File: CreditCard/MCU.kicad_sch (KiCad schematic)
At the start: 20 parts, among them J2 MEM2052-00-195-00-A_REVA, U3 PTS645SK43SMTR92LFS, U4 PTS645SK43SMTR92LFS, U8 ESP32-C6-WROOM-1U-N4, Y1 MS1V-T1K-32.768KHZ-12.5PF-20P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

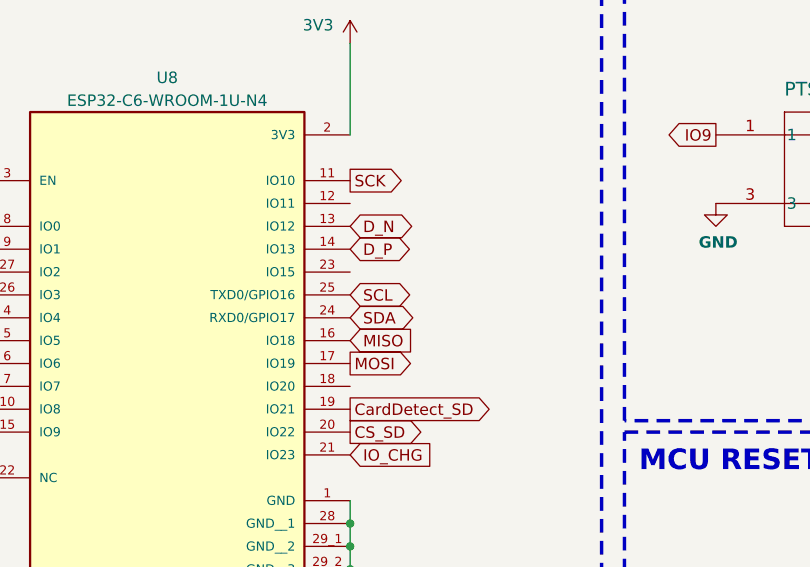
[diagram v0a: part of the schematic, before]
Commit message: connection du audio amp
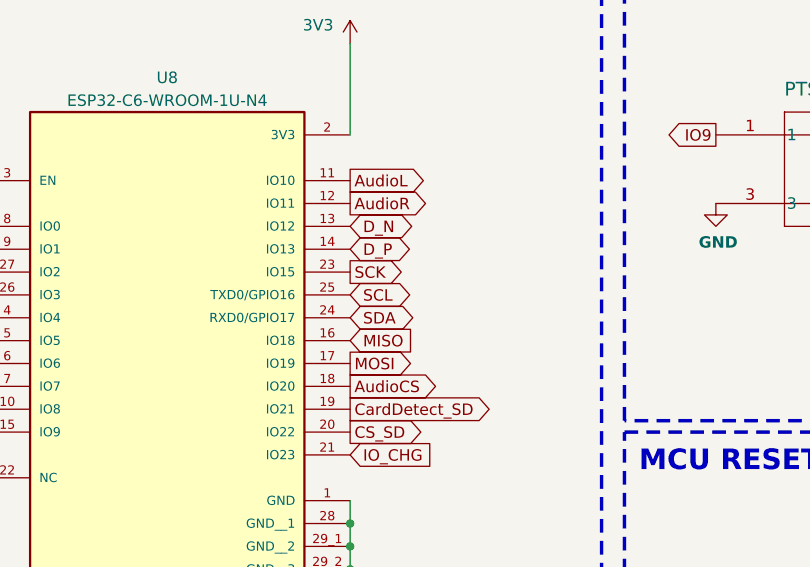
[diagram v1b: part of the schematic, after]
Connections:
- net SCK: now also U8.23 (IO15); no longer U8.11 (IO10)
- net AudioR: now reaches U8.12 (IO11)
- net AudioCS: now reaches U8.18 (IO20)
- new net AudioL: U8.11 (IO10)
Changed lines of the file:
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@@
+		)
+	)
+	(global_label "AudioL"
+		(shape output)
+		(at 185.42 48.26 0)
+		(fields_autoplaced yes)
+		(effects
+			(font
+				(size 1.27 1.27)
+			)
+			(justify left)
+		)
+		(property "Intersheetrefs" "${INTERSHEET_REFS}"
+			(at 194.5737 48.26 0)
+			(effects
+				(font
+					(size 1.27 1.27)
+				)
+				(justify left)
+				(hide yes)
+			)
 		)
 	)
@@
 		)
 	)
+	(global_label "SCK"
+		(shape output)
+		(at 185.42 58.42 0)
+		(fields_autoplaced yes)
+		(effects
+			(font
+				(size 1.27 1.27)
+			)
+			(justify left)
+		)
+		(property "Intersheetrefs" "${INTERSHEET_REFS}"
+			(at 192.1547 58.42 0)
+			(effects
+				(font
+					(size 1.27 1.27)
+				)
+				(justify left)
+				(hide yes)
+			)
+		)
+	)
 	(global_label "CardDetect_SD"
 		(shape output)
@@
 		)
 	)
+	(global_label "AudioR"
+		(shape output)
+		(at 185.42 50.8 0)
+		(fields_autoplaced yes)
+		(effects
+			(font
+				(size 1.27 1.27)
+			)
+			(justify left)
+		)
+		(property "Intersheetrefs" "${INTERSHEET_REFS}"
+			(at 194.8156 50.8 0)
+			(effects
+				(font
+					(size 1.27 1.27)
+				)
+				(justify left)
+				(hide yes)
+			)
+		)
+	)
 	(global_label "IO_CHG"
 		(shape input)
@@
 		)
 	)
-	(global_label "SCK"
-		(shape output)
-		(at 185.42 48.26 0)
-		(fields_autoplaced yes)
-		(effects
-			(font
-				(size 1.27 1.27)
-			)
-			(justify left)
-		)
-		(property "Intersheetrefs" "${INTERSHEET_REFS}"
-			(at 192.1547 48.26 0)
-			(effects
-				(font
-					(size 1.27 1.27)
-				)
-				(justify left)
-				(hide yes)
-			)
-		)
-	)
 	(global_label "MCU_EN"
 		(shape output)
@@
 				(hide yes)
 			)
+		)
+	)
+	(global_label "AudioCS"
+		(shape output)
+		(at 185.42 71.12 0)
+		(fields_autoplaced yes)
+		(effects
+			(font
+				(size 1.27 1.27)
+			)
+			(justify left)
+		)
+		(property "Intersheetrefs" "${INTERSHEET_REFS}"
+			(at 196.0251 71.12 0)
+			(effects
+				(font
+					(size 1.27 1.27)
+				)
+				(justify left)
+				(hide yes)
+			)
